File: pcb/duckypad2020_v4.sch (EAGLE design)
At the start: 98 parts, among them IC1 STM32F072C8T6, IC2 REG1117, IC3 74AHCT1G08DBV, SW1 324_SW324_SWITCH_FOOT_HOLE, SW10 KAILH_SWITCH_SOCKET_KAILH_SWI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, SW11 KAILH_SWITCH_SOCKET_KAILH_SWI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, SW12 KAILH_SWITCH_SOCKET_KAILH_SWI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, SW13 KAILH_SWITCH_SOCKET_KAILH_SWI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, SW14 KAILH_SWITCH_SOCKET_KAILH_SWI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, SW15 KAILH_SWITCH_SOCKET_KAILH_SWI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, SW16 KAILH_SWITCH_SOCKET_KAILH_SWI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, SW17 KAILH_SWITCH_SOCKET_KAILH_SWI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, SW18 KAILH_SWITCH_SOCKET_KAILH_SWI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, SW19 KAILH_SWITCH_SOCKET_KAILH_SWI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, SW2 324_SW324_SWITCH_FOOT_HOLE, SW20 SPST_TACT-EVQQ2, SW21 SPST_TACT-EVQQ2, SW5 KAILH_SWITCH_SOCKET_KAILH_SWI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, SW6 KAILH_SWITCH_SOCKET_KAILH_SWI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, SW7 KAILH_SWITCH_SOCKET_KAILH_SWI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, SW8 KAILH_SWITCH_SOCKET_KAILH_SWI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, SW9 KAILH_SWITCH_SOCKET_KAILH_SWI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, U1 UG-2864HSWEG01, U2 USBC_16P, U3 USBC_16P

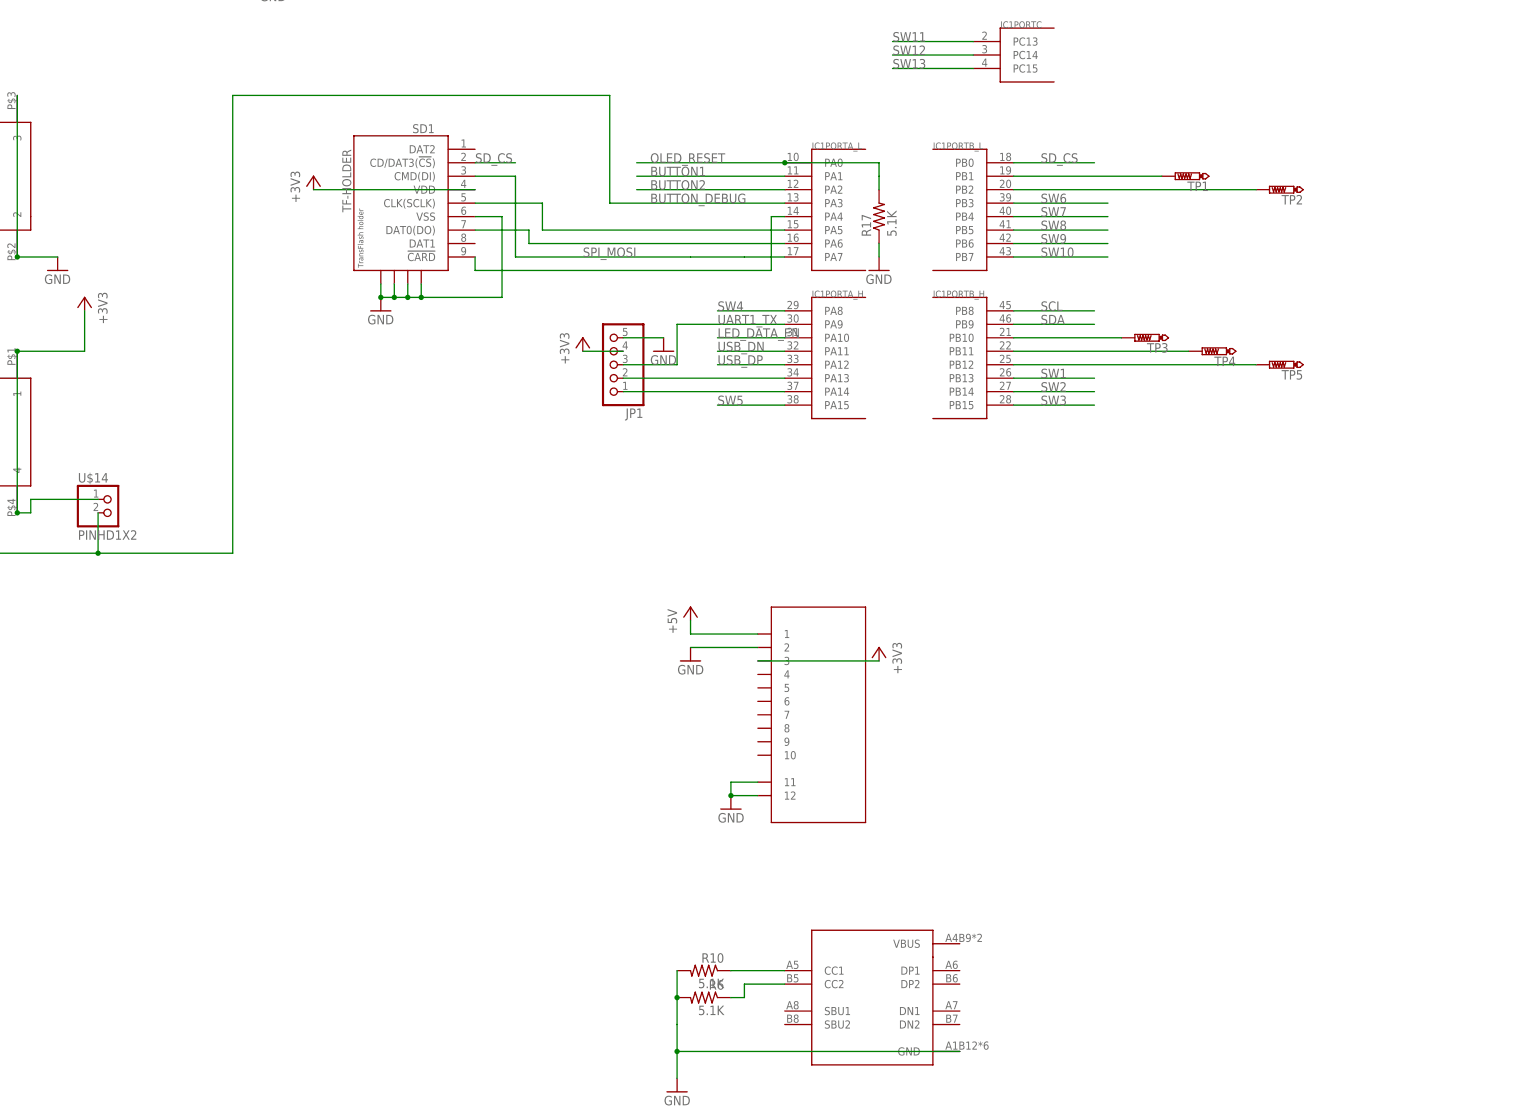
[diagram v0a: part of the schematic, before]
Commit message: v4 draft done
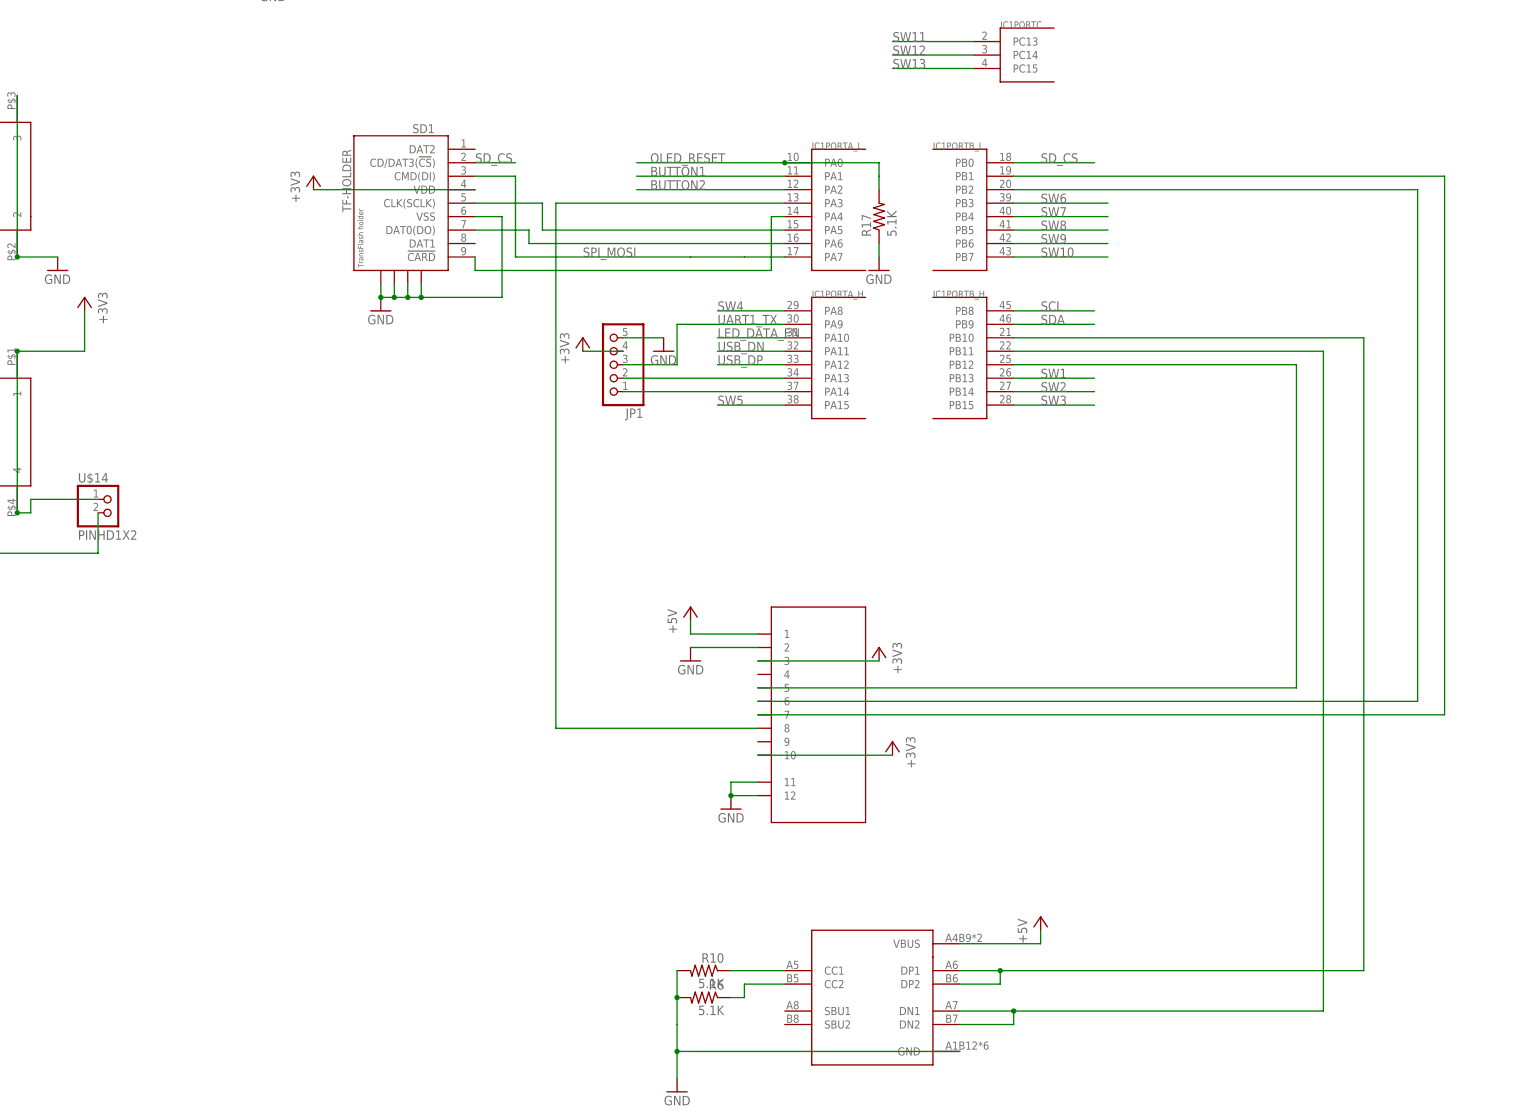
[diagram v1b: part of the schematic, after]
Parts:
- removed TP1, TP2, TP3, TP5: PTR1TP11SQ, testpad:PTR1TP11SQ
- removed TP4: PTR1TP09R, testpad:PTR1TP09R
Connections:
- new net N$37: IC1PORTA_L.PA3, SH1.8
- net +3V3: now also SH1.10
- net +5V: now also U3.VBUS
- net BUTTON_DEBUG: no longer IC1PORTA_L.PA3
- net N$13: now also IC1PORTB_L.PB1, SH1.7; no longer IC1PORTB_L.PB2, TP2.TP
- net N$16: now also IC1PORTB_H.PB11, U3.DN1, U3.DN2; no longer IC1PORTB_H.PB10, TP3.TP
- net N$2: now also IC1PORTB_L.PB2, SH1.6; no longer IC1PORTB_L.PB1, TP1.TP
- net N$30: now also IC1PORTB_H.PB10, U3.DP1, U3.DP2; no longer IC1PORTB_H.PB11, TP4.TP
- net N$35: now also SH1.5; no longer TP5.TP
